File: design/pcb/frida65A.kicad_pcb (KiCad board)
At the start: 4 copper layers, 100 x 100 mm, 105 parts, among them J1 DisplayPort Molex 472720024, J10 VIN CFG, J11 TP AMP, J12 MiniFitJr Molex 469990014, J13 POWER, J14 RJ45 Molex 446200002, J15 SPI TP, J2 TP CLOCKS, J3 SMA Molex 733910070, J4 SMA Molex 733910070, J5 DIFF/SE CFG, J6 TERM CFG, J7 ATTEN CFG, J8 SMA Molex 733910070, J9 TERM CFG, Q1 Q_PMOS_DGS, U1 DiffAmp TI THS4541, U2 TI LevelShifter SN74AXC8T245R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, U3 ASIC FRIDA 65A

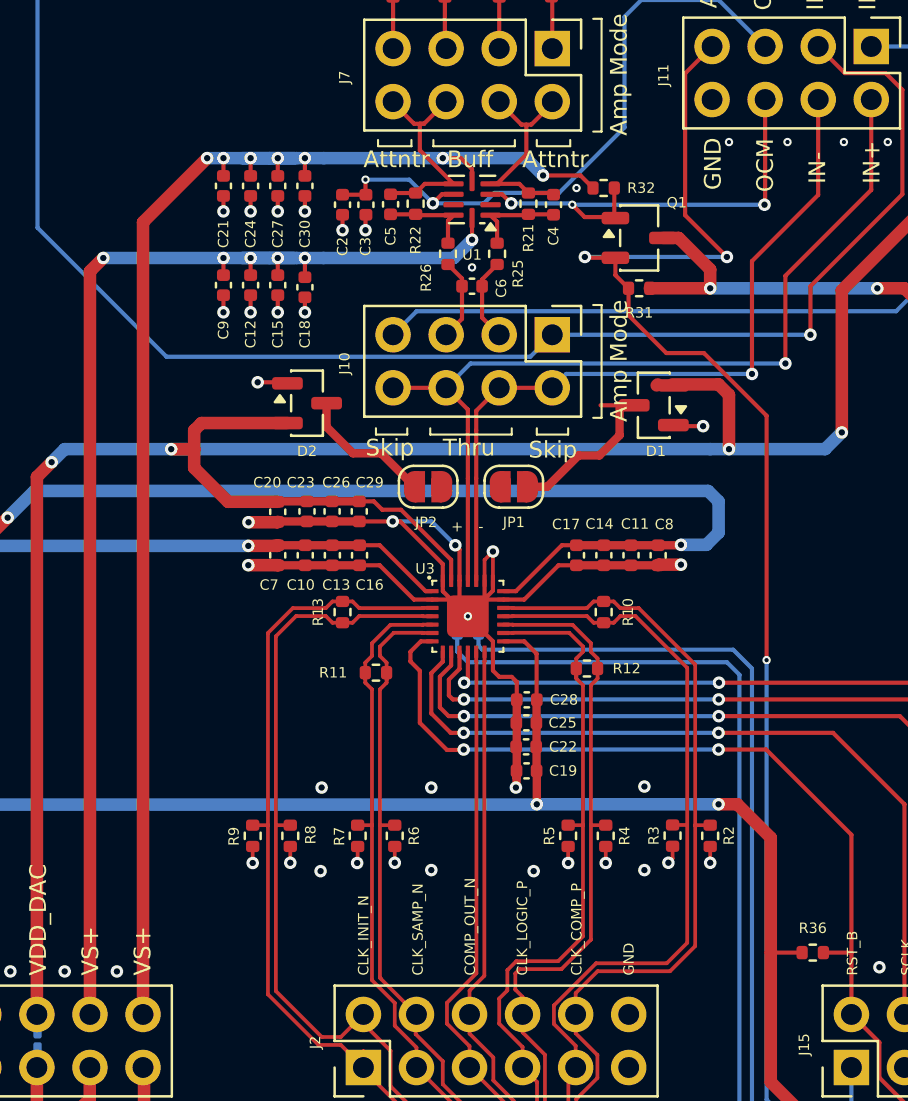
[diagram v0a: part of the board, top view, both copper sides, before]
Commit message: chore(pcb): update schematic and layout
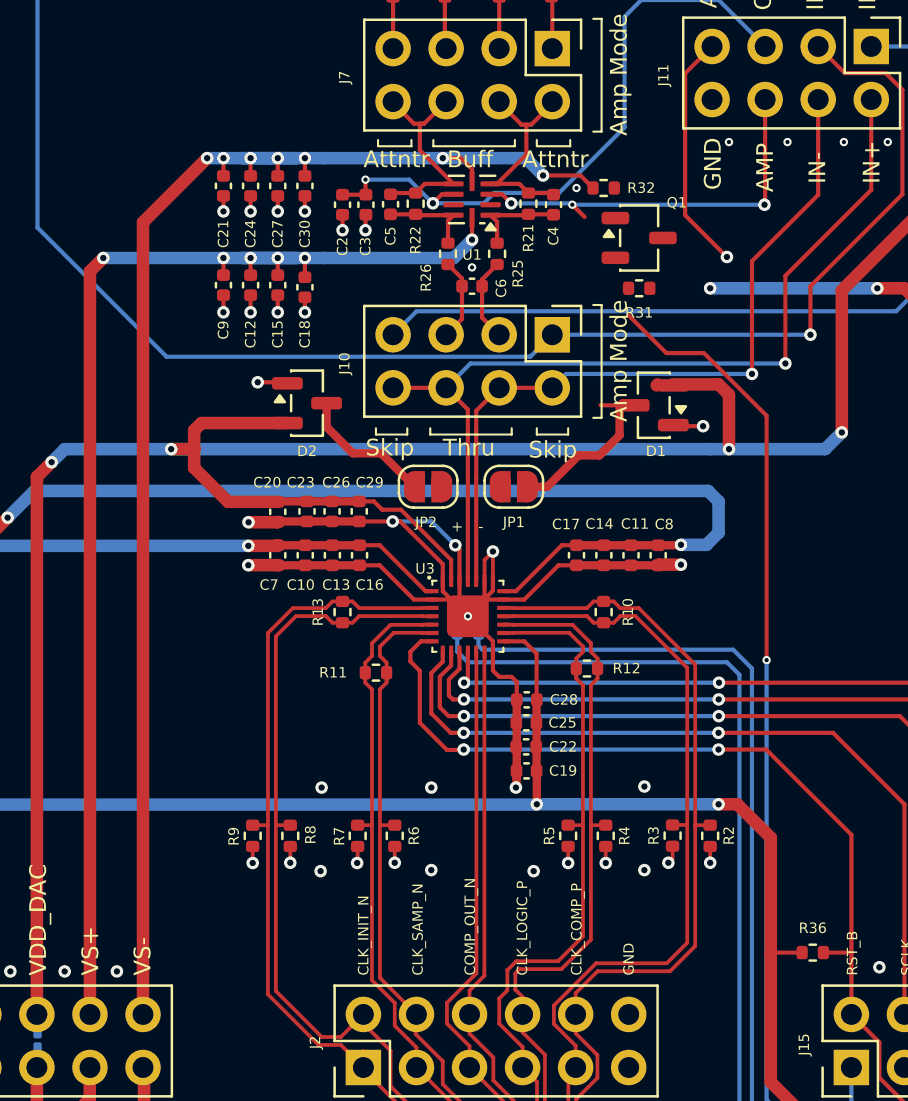
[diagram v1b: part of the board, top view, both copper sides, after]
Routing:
- net /AMP_PD_EXT: track 84.7 -> 73.4 mm, vias 4 -> 3
- net /VDD_BDAQ: track 112.2 -> 105.5 mm
- net /AMP_PD_N: track 22.2 -> 19.3 mm
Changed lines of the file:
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@@
 		)
 	)
-	(gr_text "OCM"
+	(gr_text "AMP"
 		(at 164.7 79.6 90)
 		(layer "F.SilkS")
@@
 		)
 	)
-	(gr_text "VS+"
+	(gr_text "VS-"
 		(at 134.9 117.1 90)
 		(layer "F.SilkS")
@@
 	)
 	(segment
-		(start 161.6 84.2)
-		(end 158.71 84.2)
-		(width 0.6)
-		(layer "F.Cu")
-		(net 58)
-	)
-	(segment
-		(start 160.09 81.79)
-		(end 159.3375 81.79)
-		(width 0.6)
-		(layer "F.Cu")
-		(net 58)
-	)
-	(segment
 		(start 172.11 128.29)
 		(end 173 128.29)
@@
 	)
 	(segment
-		(start 161.6 84.2)
-		(end 161.6 83.3)
-		(width 0.6)
-		(layer "F.Cu")
-		(net 58)
-	)
-	(segment
-		(start 161.6 83.3)
-		(end 160.09 81.79)
-		(width 0.6)
-		(layer "F.Cu")
-		(net 58)
-	)
-	(segment
 		(start 170.38 130.4)
 		(end 171.388 130.4)
@@
 	)
 	(segment
-		(start 155.64 82.74)
-		(end 155.6 82.7)
-		(width 0.2)
-		(layer "F.Cu")
-		(net 59)
-	)
-	(segment
 		(start 160.4 73.915)
 		(end 161.69 72.625)
@@
 	)
 	(segment
-		(start 157.69 85.49)
-		(end 157.69 84.2)
-		(width 0.2)
-		(layer "F.Cu")
-		(net 59)
-	)
-	(segment
 		(start 161.3 87.3)
 		(end 159.5 87.3)
@@
 	)
 	(segment
-		(start 157.0625 82.74)
-		(end 155.64 82.74)
-		(width 0.2)
-		(layer "F.Cu")
-		(net 59)
-	)
-	(segment
 		(start 159.5 87.3)
 		(end 157.69 85.49)
@@
 	)
 	(segment
-		(start 157.0625 83.5725)
-		(end 157.69 84.2)
-		(width 0.2)
-		(layer "F.Cu")
-		(net 59)
-	)
-	(segment
 		(start 173.42 139.8585)
 		(end 173.42 132.42)
@@
 		(net 59)
 	)
-	(segment
-		(start 157.0625 82.74)
-		(end 157.0625 83.5725)
-		(width 0.2)
-		(layer "F.Cu")
-		(net 59)
-	)
-	(via
-		(at 155.6 82.7)
-		(size 0.6)
-		(drill 0.3)
-		(layers "F.Cu" "B.Cu")
-		(net 59)
-	)
 	(via
 		(at 162.4 82.7)
@@
 	)
 	(segment
-		(start 155.6 82.7)
-		(end 162.4 82.7)
-		(width 0.2)
-		(layer "B.Cu")
-		(net 59)
-	)
-	(segment
 		(start 164.3 123.041479)
 		(end 164.3 102)
@@
 		(width 0.2)
 		(layer "F.Cu")
-		(net 60)
-	)
-	(segment
-		(start 157.0125 80.79)
-		(end 155.59 80.79)
-		(width 0.2)
-		(layer "F.Cu")
-		(net 60)
-	)
-	(segment
-		(start 157.01 79.4)
-		(end 157.01 80.7875)
-		(width 0.2)
-		(layer "F.Cu")
